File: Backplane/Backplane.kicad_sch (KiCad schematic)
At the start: 15 parts

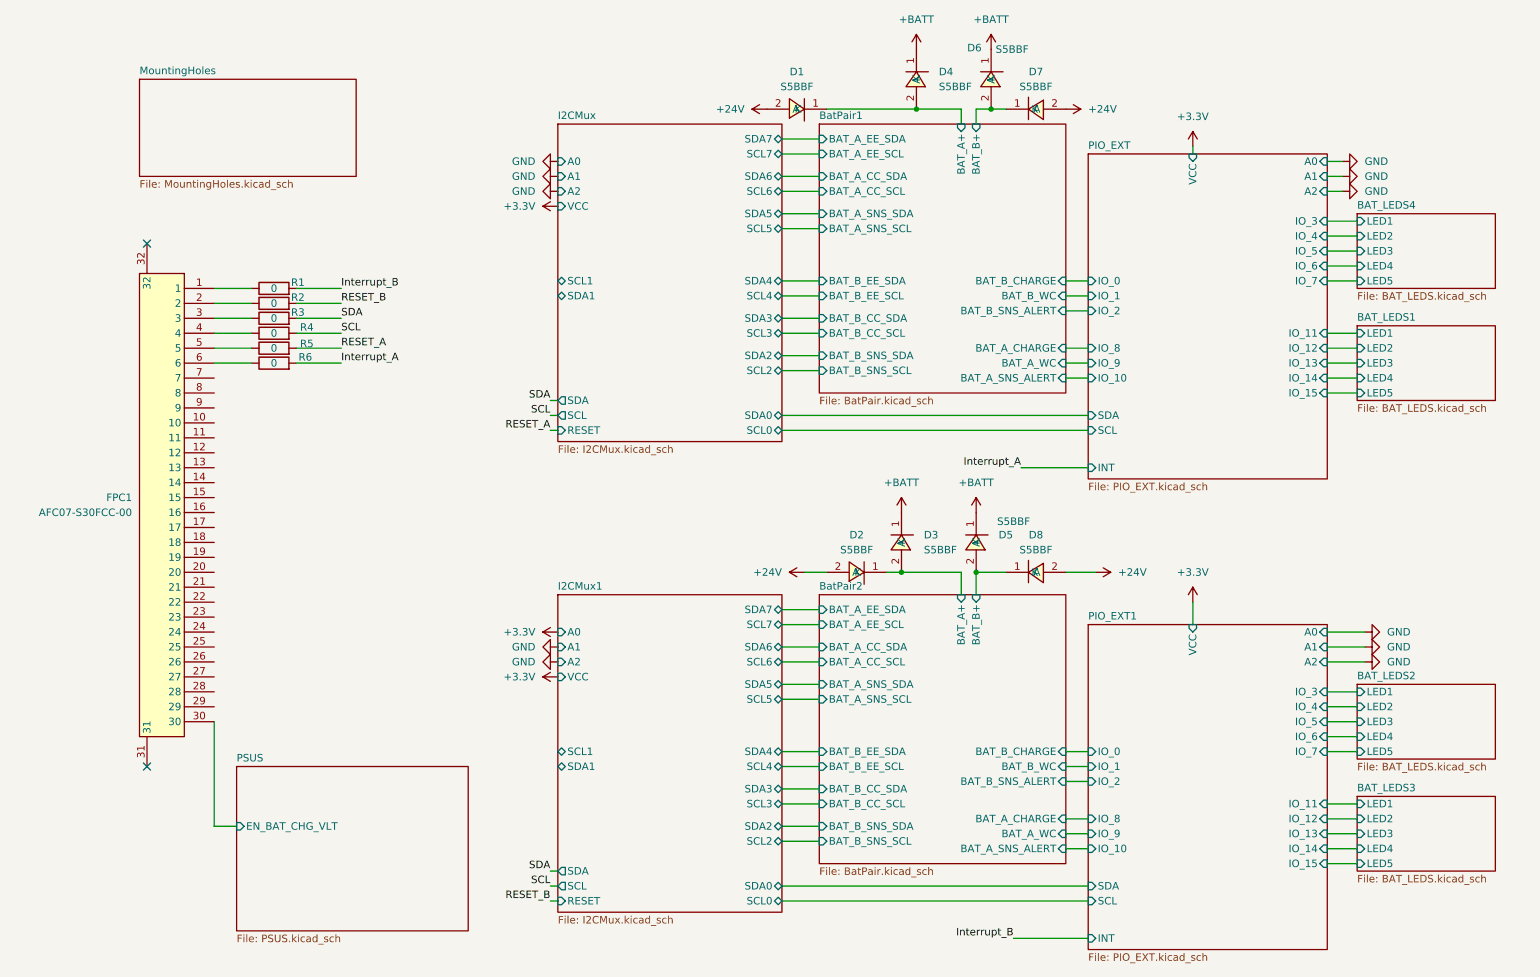
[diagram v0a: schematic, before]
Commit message: added
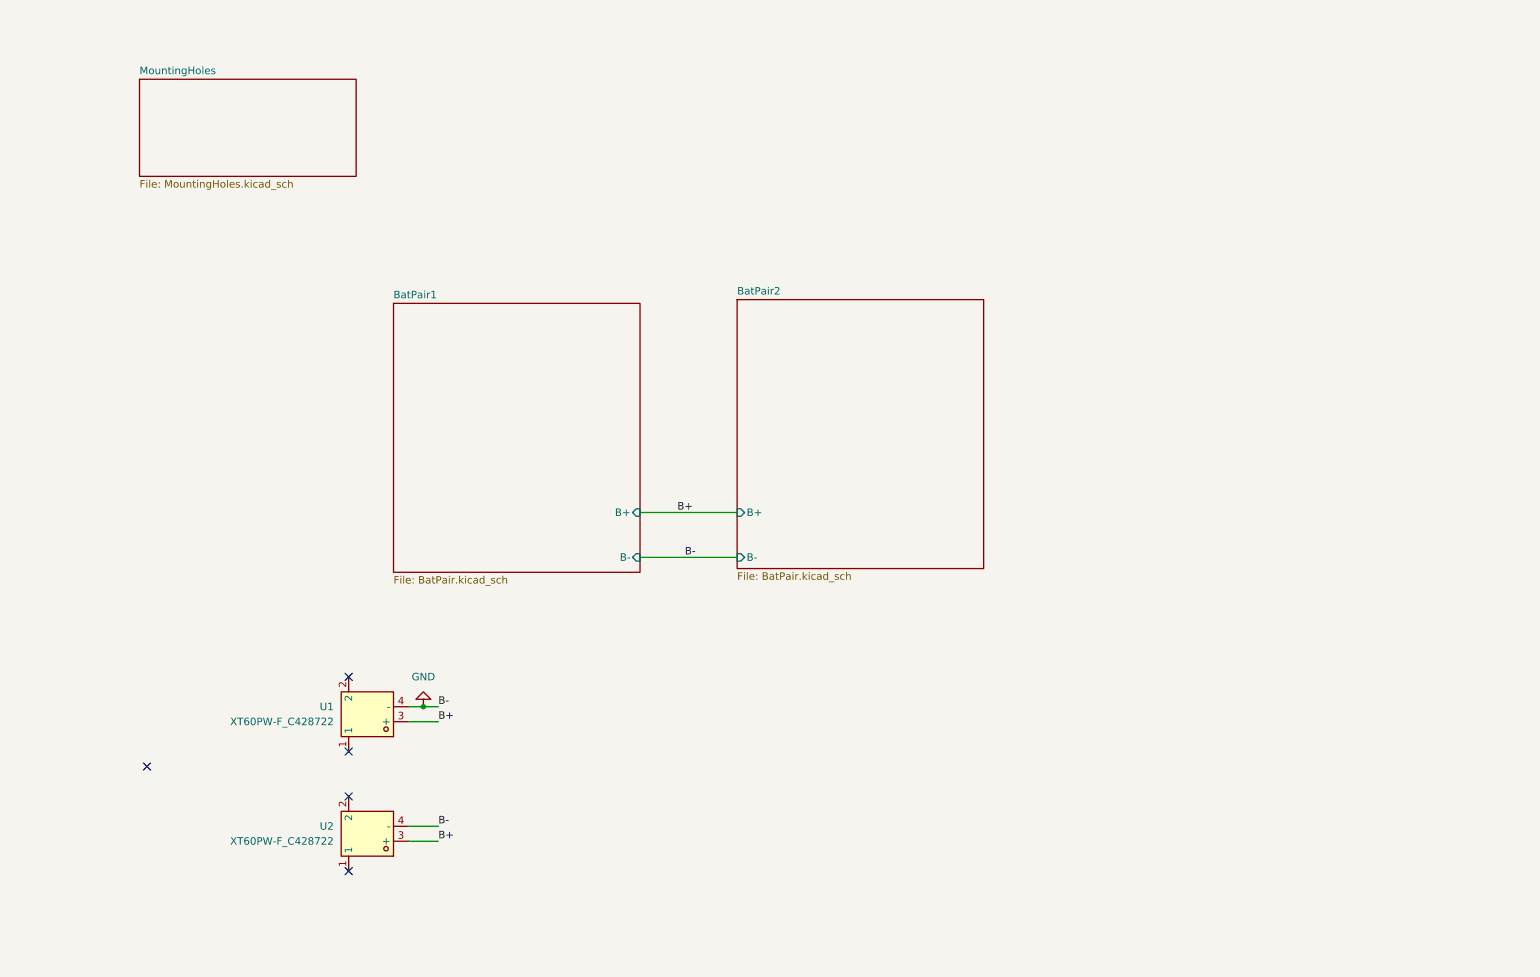
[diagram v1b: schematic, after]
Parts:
- removed D1, D2, D3, D4, D5, D6, D7, D8: S5BBF, COMPONENTS:SMBF_L4.3-W3.6-LS5.3-RD, symbol COMPONENTS:S5BBF
- removed FPC1: AFC07-S30FCC-00, COMPONENTS:FPC-SMD_P0.50-30P_LCSXJ-H2.0, symbol COMPONENTS:AFC07-S30FCC-00
- removed R1, R2, R3, R4, R5, R6: 0, Resistor_SMD:R_1206_3216Metric_Pad1.30x1.75mm_HandSolder, symbol Device:R
- added U1, U2: XT60PW-F_C428722, COMPONENTS:TH_2P-XT60PW-F, symbol COMPONENTS:XT60PW-F_C428722
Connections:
- net GND: now also U1.4 (-), U2.4 (-)
- new net B+: U1.3 (+), U2.3 (+)
- no-connect marks 2 -> 5
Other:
- removed sheet BAT_LEDS1
- removed sheet BAT_LEDS2
- removed sheet BAT_LEDS3
- removed sheet BAT_LEDS4
- removed sheet I2CMux
- removed sheet I2CMux1
- removed sheet PIO_EXT
- removed sheet PIO_EXT1
- removed sheet PSUS
- sheet BatPair1 ports: added B+, B-; removed BAT_A+, BAT_A_CC_SCL, BAT_A_CC_SDA, BAT_A_CHARGE, BAT_A_EE_SCL, BAT_A_EE_SDA, BAT_A_SNS_ALERT, BAT_A_SNS_SCL, BAT_A_SNS_SDA, BAT_A_WC, BAT_B+, BAT_B_CC_SCL, BAT_B_CC_SDA, BAT_B_CHARGE, BAT_B_EE_SCL, BAT_B_EE_SDA, BAT_B_SNS_ALERT, BAT_B_SNS_SCL, BAT_B_SNS_SDA, BAT_B_WC
- sheet BatPair2 ports: added B+, B-; removed BAT_A+, BAT_A_CC_SCL, BAT_A_CC_SDA, BAT_A_CHARGE, BAT_A_EE_SCL, BAT_A_EE_SDA, BAT_A_SNS_ALERT, BAT_A_SNS_SCL, BAT_A_SNS_SDA, BAT_A_WC, BAT_B+, BAT_B_CC_SCL, BAT_B_CC_SDA, BAT_B_CHARGE, BAT_B_EE_SCL, BAT_B_EE_SDA, BAT_B_SNS_ALERT, BAT_B_SNS_SCL, BAT_B_SNS_SDA, BAT_B_WC
